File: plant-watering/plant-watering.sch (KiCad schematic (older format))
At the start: 1 part, among them U1 ESP32-DEVKITC-32D

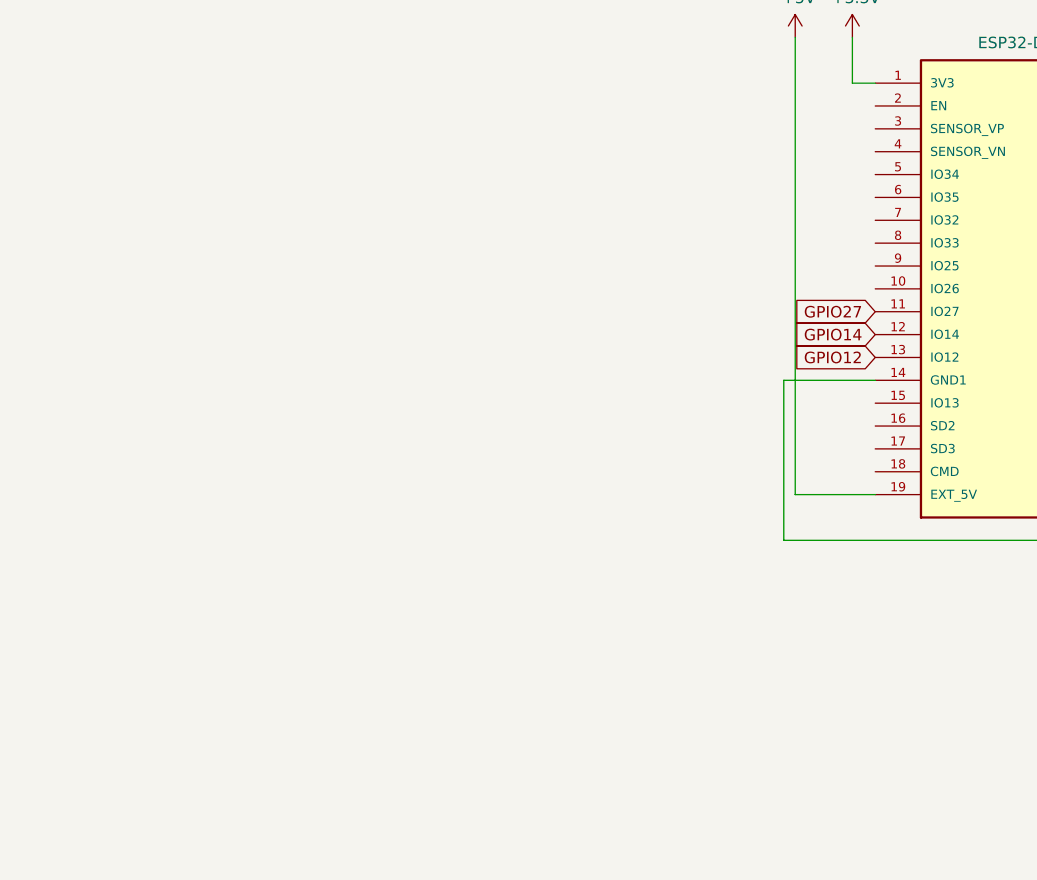
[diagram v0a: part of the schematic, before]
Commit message: added many schematicy
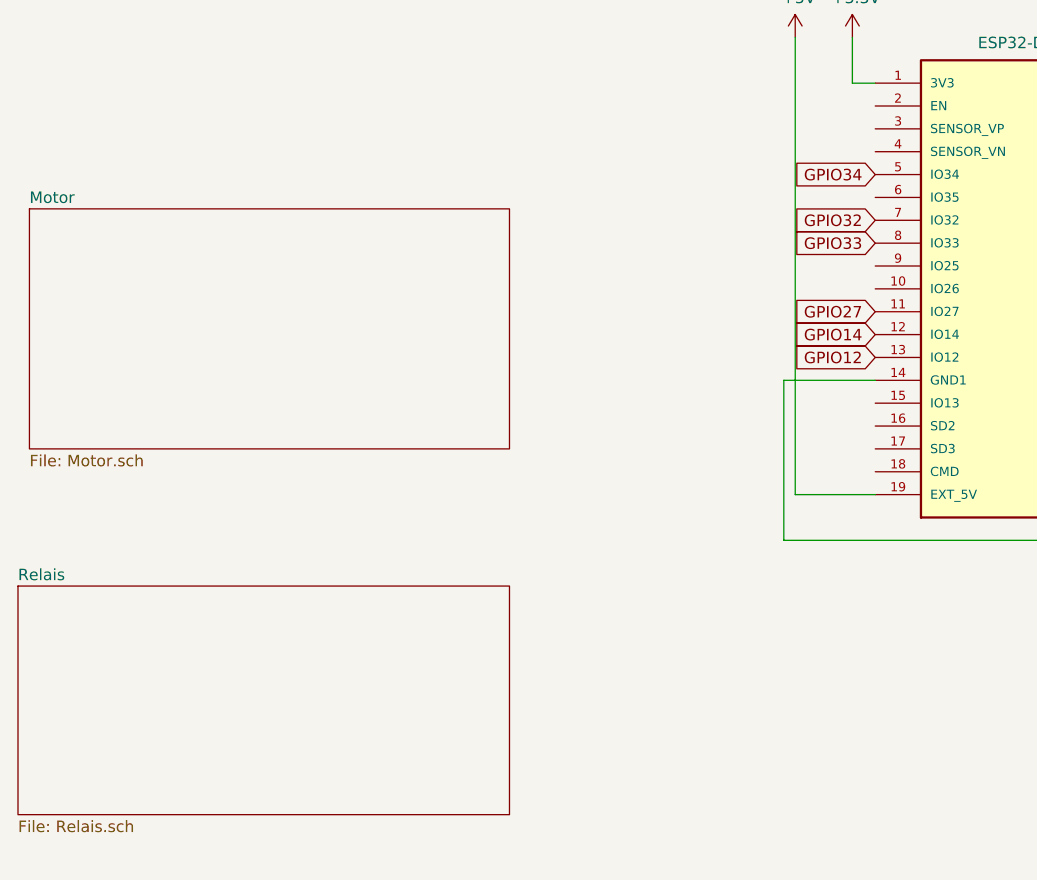
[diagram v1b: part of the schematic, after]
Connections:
- net GPIO34: now reaches U1.5 (IO34)
- net GPIO32: now reaches U1.7 (IO32)
- net GPIO33: now reaches U1.8 (IO33)
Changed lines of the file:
@@
 $Descr A4 11693 8268
 encoding utf-8
-Sheet 1 4
+Sheet 1 6
 Title ""
 Date "2021-01-20"
@@
 F1 "Input.sch" 50
 $EndSheet
+Text GLabel 4450 3100 0    50   Input ~ 0
+GPIO32
+Text GLabel 4450 3200 0    50   Input ~ 0
+GPIO33
+Text GLabel 4450 2900 0    50   Input ~ 0
+GPIO34
+$Sheet
+S 700  4700 2150 1000
+U 600A014F
+F0 "Relais" 50
+F1 "Relais.sch" 50
+$EndSheet
+$Sheet
+S 750  3050 2100 1050
+U 600B5D96
+F0 "Motor" 50
+F1 "Motor.sch" 50
+$EndSheet
 $EndSCHEMATC

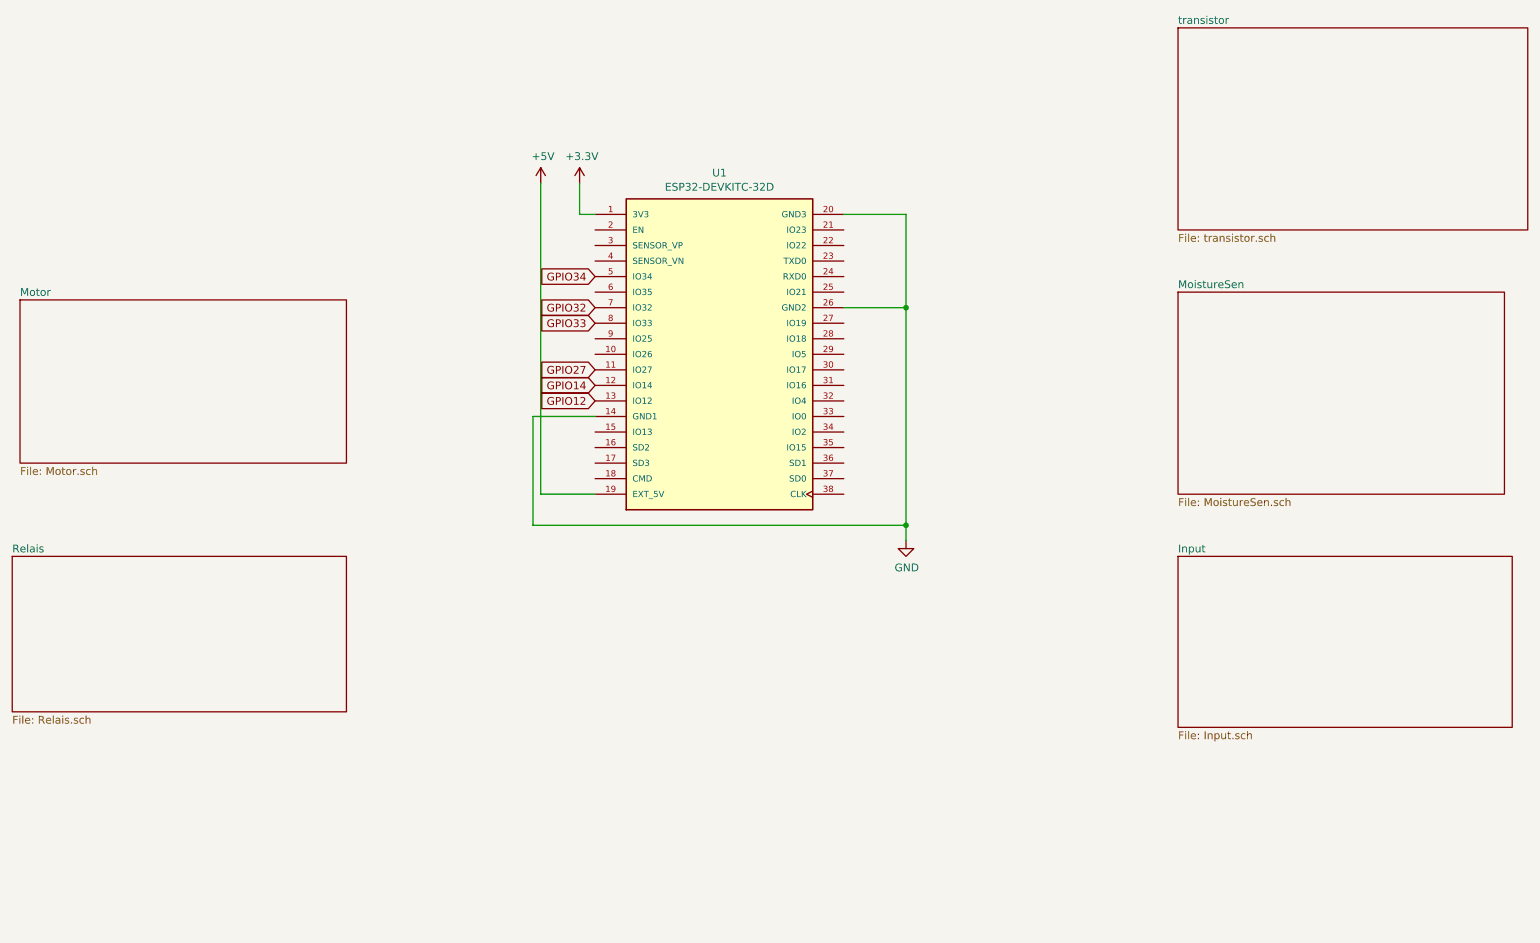
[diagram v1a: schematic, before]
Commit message: added several parts#
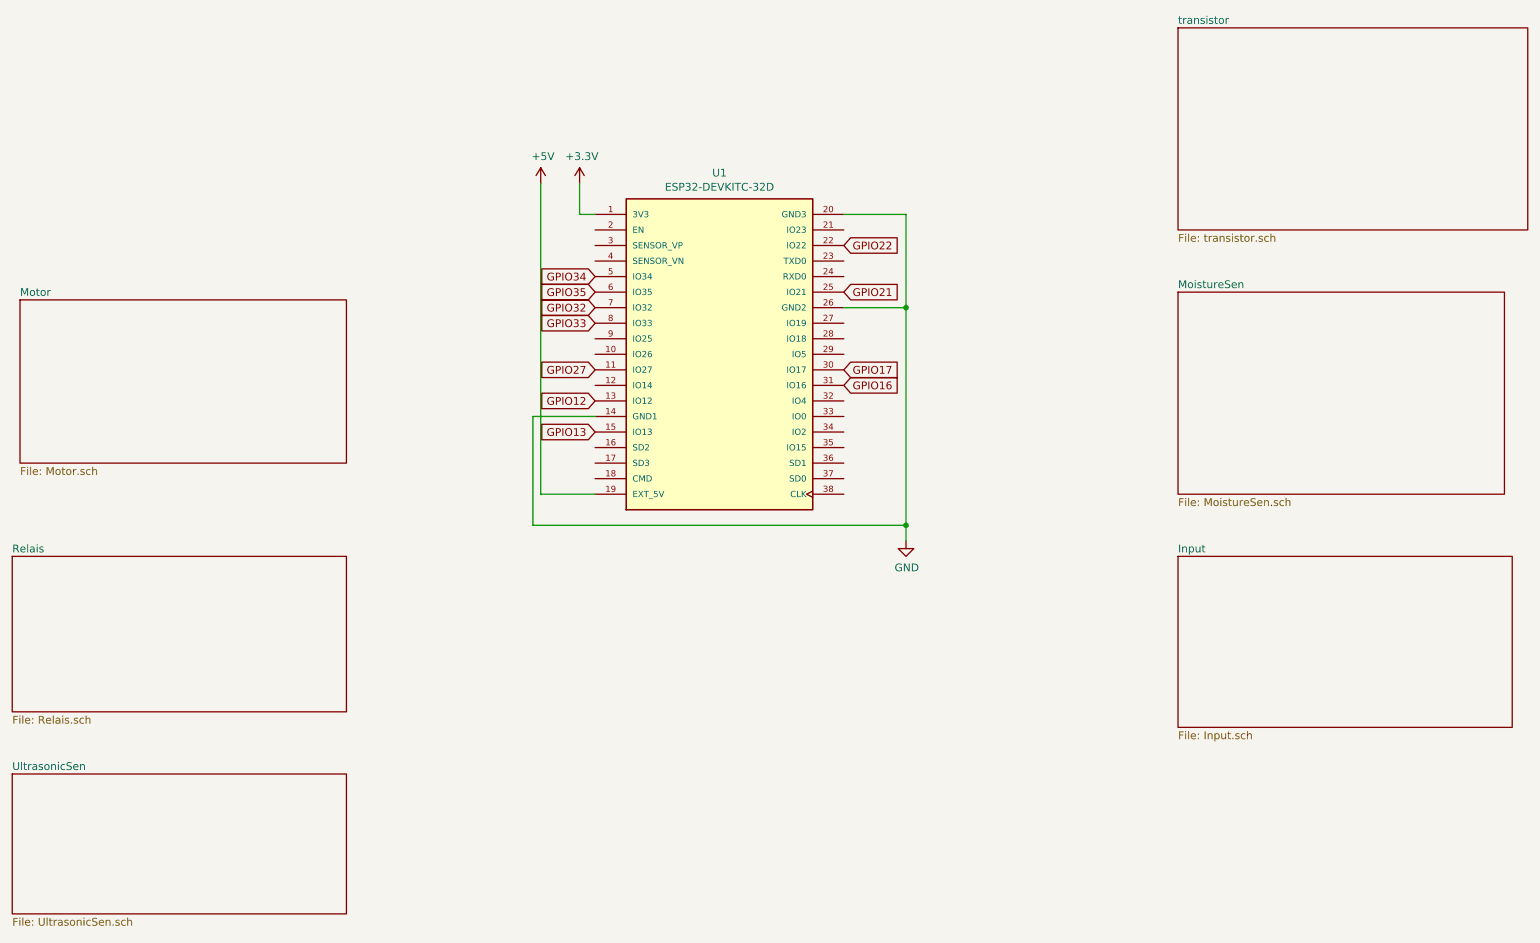
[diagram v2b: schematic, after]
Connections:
- net GPIO13: now reaches U1.15 (IO13)
- net GPIO22: now reaches U1.22 (IO22)
- net GPIO21: now reaches U1.25 (IO21)
- net GPIO17: now reaches U1.30 (IO17)
- net GPIO16: now reaches U1.31 (IO16)
- net GPIO35: now reaches U1.6 (IO35)
- net GPIO14: no longer names the net of U1.12 (IO14)
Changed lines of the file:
@@
 $Descr A4 11693 8268
 encoding utf-8
-Sheet 1 6
+Sheet 1 7
 Title ""
 Date "2021-01-20"
@@
 Text GLabel 4450 3700 0    50   Input ~ 0
 GPIO12
-Text GLabel 4450 3600 0    50   Input ~ 0
-GPIO14
+Text GLabel 4450 3900 0    50   Input ~ 0
+GPIO13
 Text GLabel 4450 3500 0    50   Input ~ 0
 GPIO27
@@
 F1 "Motor.sch" 50
 $EndSheet
+$Sheet
+S 700  6100 2150 900
+U 600DE063
+F0 "UltrasonicSen" 50
+F1 "UltrasonicSen.sch" 50
+$EndSheet
+Text GLabel 6050 3500 2    50   Input ~ 0
+GPIO17
+Text GLabel 6050 3600 2    50   Input ~ 0
+GPIO16
+Text GLabel 6050 2700 2    50   Input ~ 0
+GPIO22
+Text GLabel 6050 3000 2    50   Input ~ 0
+GPIO21
+Text GLabel 4450 3000 0    50   Input ~ 0
+GPIO35
 $EndSCHEMATC

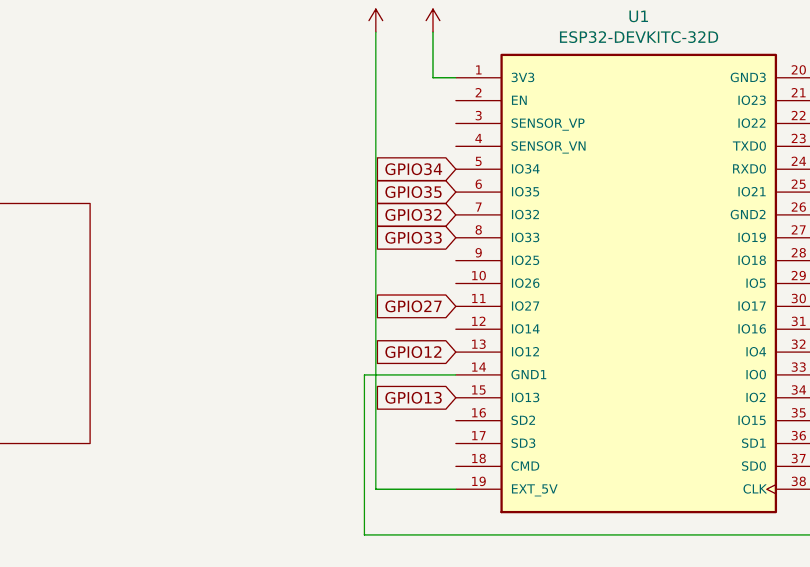
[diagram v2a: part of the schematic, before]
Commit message: finished pcb for now
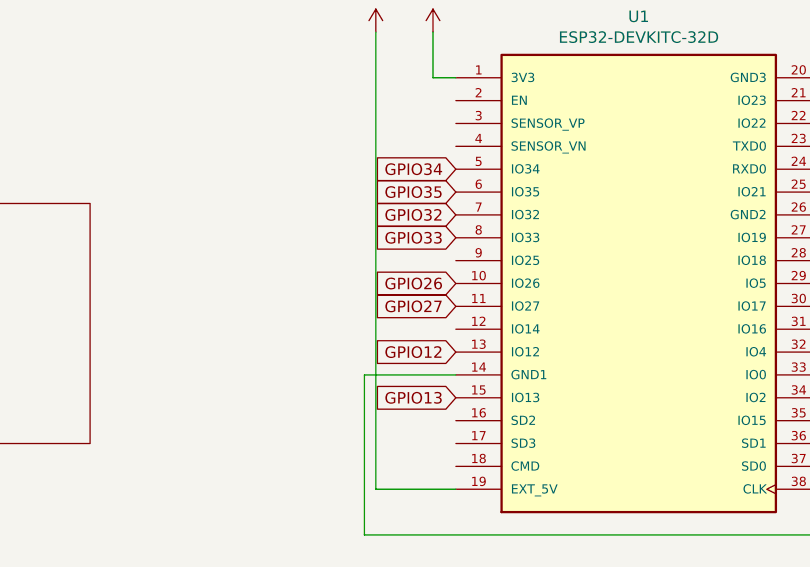
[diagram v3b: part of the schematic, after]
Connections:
- net GPIO26: now reaches U1.10 (IO26)
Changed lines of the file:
@@
 Text GLabel 4450 3000 0    50   Input ~ 0
 GPIO35
+Text GLabel 4450 3400 0    50   Input ~ 0
+GPIO26
 $EndSCHEMATC
